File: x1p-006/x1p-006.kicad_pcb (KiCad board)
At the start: 2 copper layers, 26 x 32.6 mm, 13 parts, among them U1 AD24C02, U2 TLP240A(TP1,F, U3 TLP240A(TP1,F

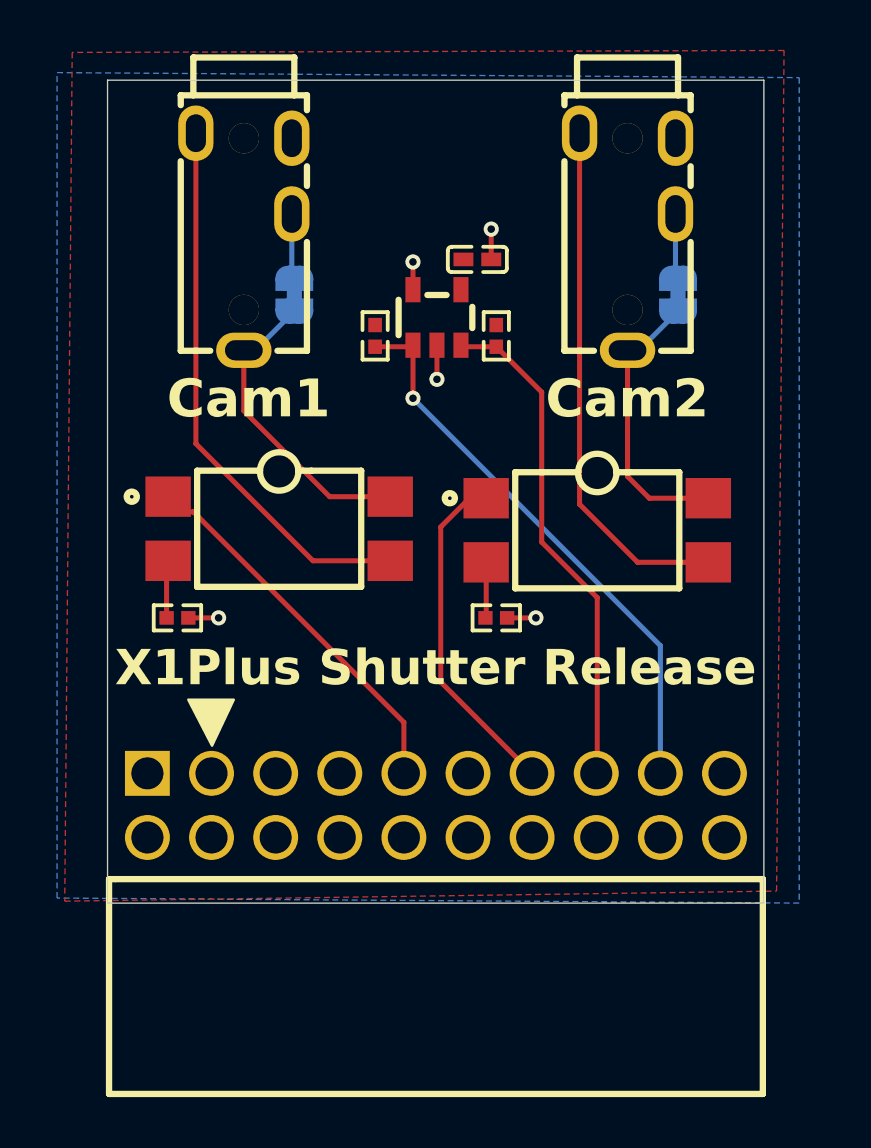
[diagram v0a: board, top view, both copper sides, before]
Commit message: fixes
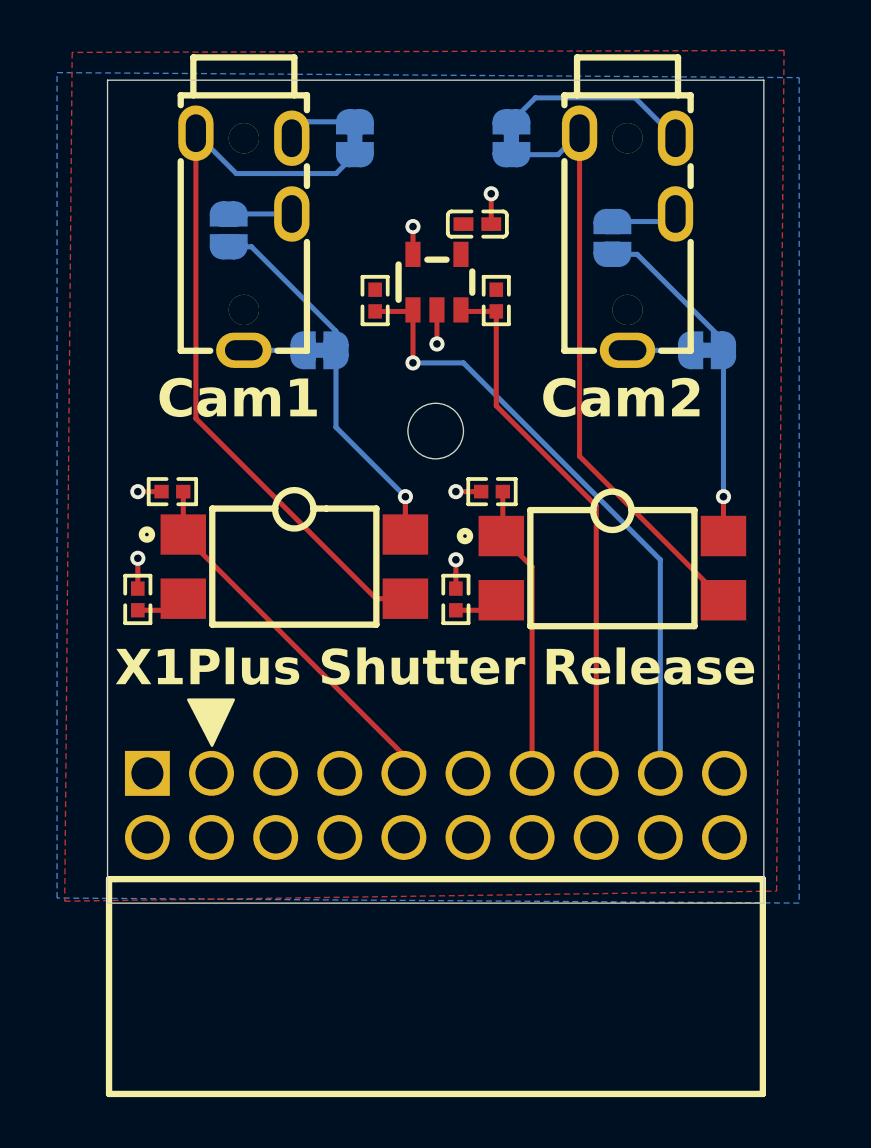
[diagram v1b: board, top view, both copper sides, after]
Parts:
- added H1: MountingHole, MountingHole:MountingHole_2.2mm_M2_ISO7380, F.Cu at (68.4, 107.8)
- added JP3: SolderJumper_2_Bridged, Jumper:SolderJumper-2_P1.3mm_Bridged_RoundedPad1.0x1.5mm, B.Cu at (65.2, 96.2)
- added JP4: SolderJumper_2_Bridged, Jumper:SolderJumper-2_P1.3mm_Bridged_RoundedPad1.0x1.5mm, B.Cu at (71.4, 96.2)
- added JP5: SolderJumper_2_Bridged, Jumper:SolderJumper-2_P1.3mm_Bridged_RoundedPad1.0x1.5mm, B.Cu at (63.8, 104.6)
- added JP6: SolderJumper_2_Bridged, Jumper:SolderJumper-2_P1.3mm_Bridged_RoundedPad1.0x1.5mm, B.Cu at (79.2, 104.6)
- added R5: 3.3k, x1p-006:R0402, F.Cu at (58.0, 110.2)
- added R6: 3.3k, x1p-006:R0402, F.Cu at (70.6, 110.2)
- JP1, JP2: value SolderJumper_2_Bridged -> SolderJumper_2_Open; footprint Jumper:SolderJumper-2_P1.3mm_Bridged_RoundedPad1.0x1.5mm -> Jumper:SolderJumper-2_P1.3mm_Open_RoundedPad1.0x1.5mm
- moved JP1 3.64 mm to (60.2, 99.8)
- moved JP2 3.44 mm to (75.4, 100.2)
- moved R4 1.76 mm to (69.2, 114.5), turned to -90 degrees
- moved R3 1.73 mm to (56.6, 114.5), turned to -90 degrees
- moved U3 1.62 mm to (75.4, 113.2)
- moved U2 1.62 mm to (62.8, 113.2)
- moved C1 1.40 mm to (70.0, 99.6)
- moved R1 1.40 mm to (66.0, 102.6)
- moved R2 1.40 mm to (70.8, 102.6)
- moved U1 1.40 mm to (68.5, 101.9)
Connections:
- CAM1 pad 2: unconnected-(CAM1-Pad2) -> Net-(JP3-B)
- CAM1 pad 4: Net-(JP1-A) -> Net-(JP5-B)
- CAM2 pad 2: unconnected-(CAM2-Pad2) -> Net-(JP4-B)
- CAM2 pad 4: Net-(JP2-A) -> Net-(JP6-B)
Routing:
- net Net-(JP3-A): track 21.7 -> 29.8 mm
- net Net-(JP4-B): track 0.00 -> 7.56 mm
- net Net-(JP4-A): track 20.8 -> 25.0 mm
- net Net-(JP3-B): track 0.00 -> 3.47 mm
- net Net-(JP1-A): track 12.1 -> 14.8 mm, vias 0 -> 1
- net Net-(JP6-B): track 0.00 -> 2.60 mm
- net Net-(JP5-B): track 0.00 -> 2.60 mm
- net LD7: track 22.5 -> 25.1 mm
- net Net-(JP2-A): track 11.2 -> 13.6 mm, vias 0 -> 1
- net GND: track 5.99 -> 7.93 mm, vias 5 -> 7
- net LD6: track 20.0 -> 21.4 mm
- net LD5: track 13.5 -> 12.4 mm
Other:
- board text added: "R"
- board text added: "S"
- board text added: "T"
